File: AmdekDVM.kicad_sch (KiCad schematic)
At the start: 59 parts, among them J1 TO_DAUGHTERBOARD, J2 VIDEO, J3 APPLE II, U1 74LS123, U10 74LS04, U11 74LS74, U12 74LS04, U13 74LS10, U14 74LS10, U15 74LS10, U16 74LS08, U17 74LS11, U18 74LS08, U19 74LS04, U2 74LS175, U20 74LS51, U21 74LS95, U22 74LS164, U23 74LS95, U24 74LS00, U25 74LS54N, U26 74LS21, U27 74LS21, U28 74LS95, U29 74LS54N, U3 74LS157, U30 74LS54N, U31 74LS04, U32 74LS259, U33 74LS02, U34 74LS51, U35 74LS30, U36 74LS04, U37 74LS08, U38 74LS30, U4 74LS175, U5 SPARE, U6 74LS95, U7 74LS95, U8 74LS95, U9 74LS164

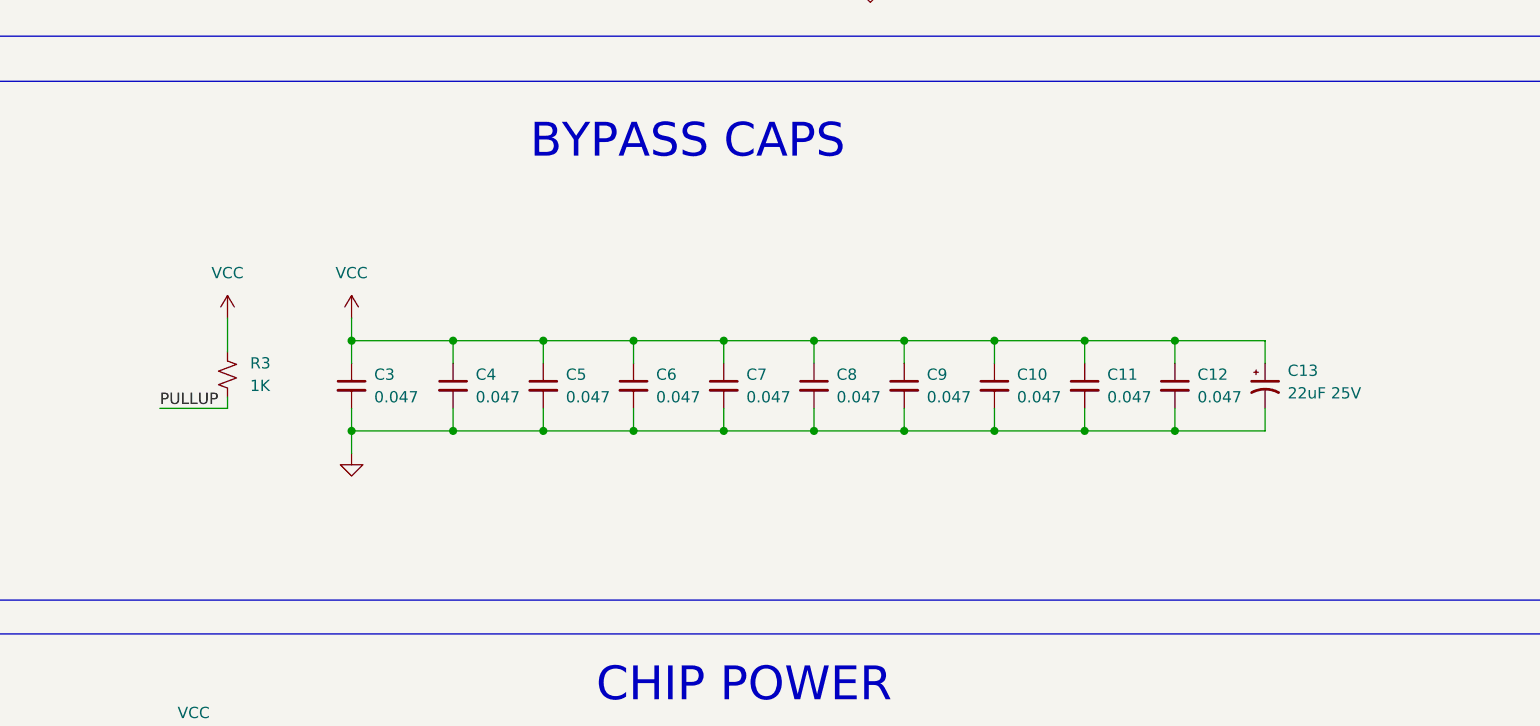
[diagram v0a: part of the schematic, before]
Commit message: Add cable details, fab packages, instructions
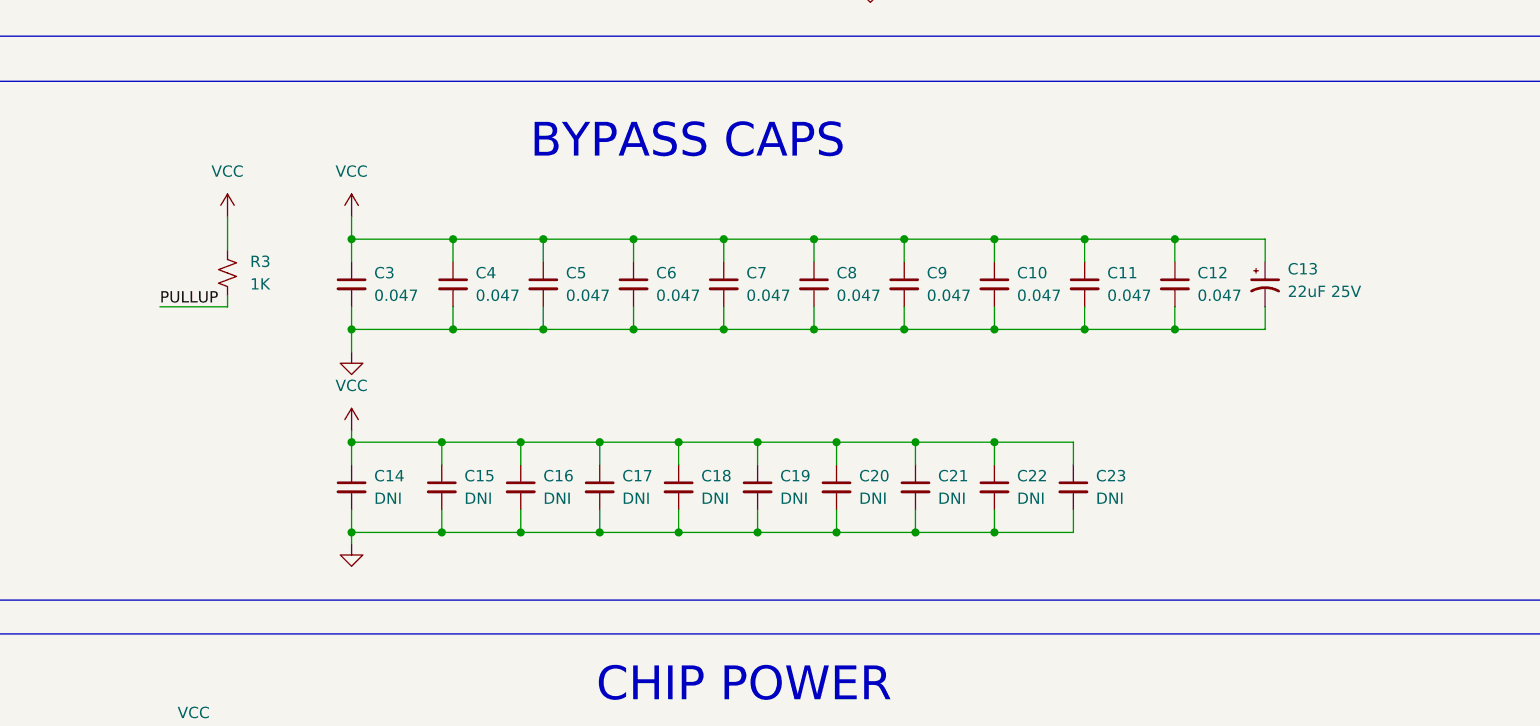
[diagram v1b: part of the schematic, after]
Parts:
- added C14, C15, C16, C17, C18, C19, C20, C21, C22, C23: DNI, Capacitor_THT:C_Disc_D4.3mm_W1.9mm_P5.00mm, symbol Device:C_Small
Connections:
- net GND: now also C14.2, C15.2, C16.2, C17.2, C18.2, C19.2, C20.2, C21.2, C22.2, C23.2
- net VCC: now also C14.1, C15.1, C16.1, C17.1, C18.1, C19.1, C20.1, C21.1, C22.1, C23.1
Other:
- moved on the sheet: C10, C11, C12, C13, C3, C4, C5, C6, C7, C8, C9, R3
